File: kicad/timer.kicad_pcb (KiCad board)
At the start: 2 copper layers, 35.1 x 40 mm, 27 parts, among them IC1 STM8S003F3P, J1 PISK, J2 USB_OTG, J3 CONN_01X02, P1 kn1, P2 bat, P3 kn1, Q4 Q_NMOS_GSD, U1 TP4056

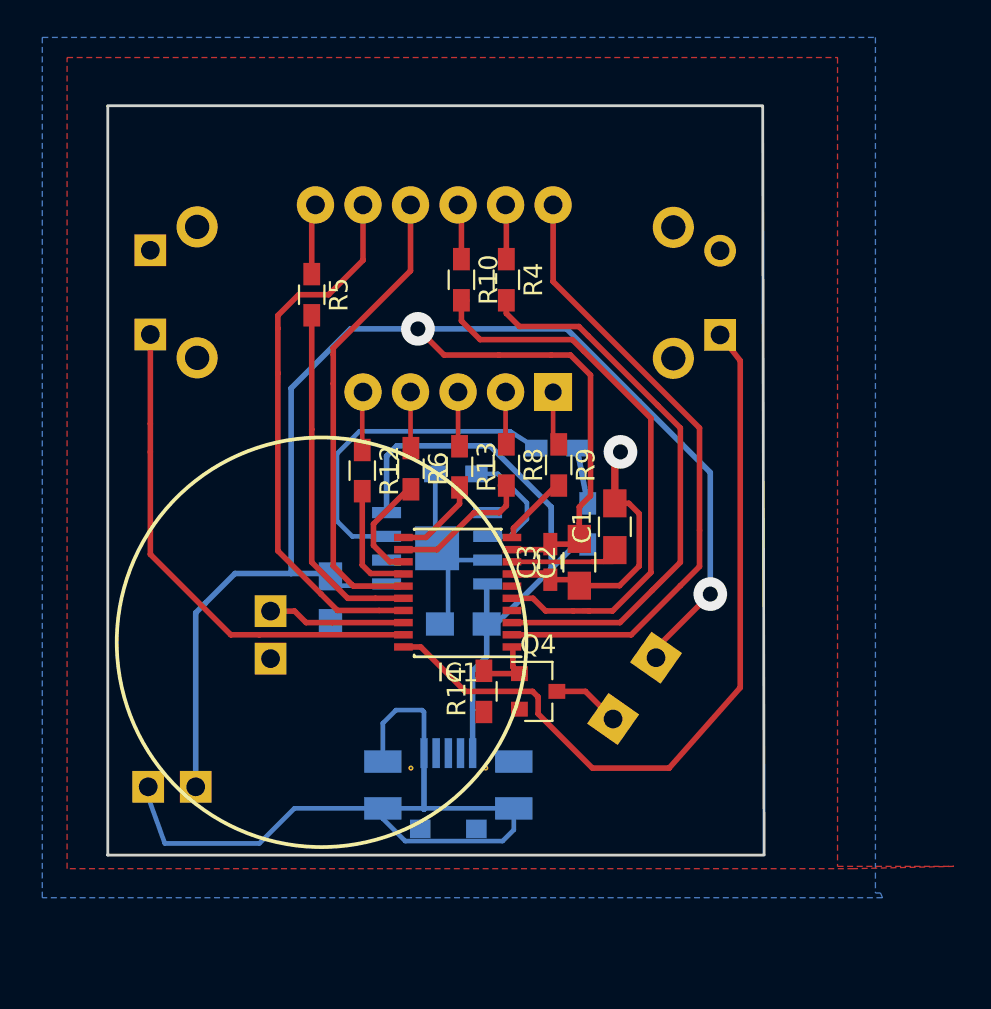
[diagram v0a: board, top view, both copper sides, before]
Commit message: start
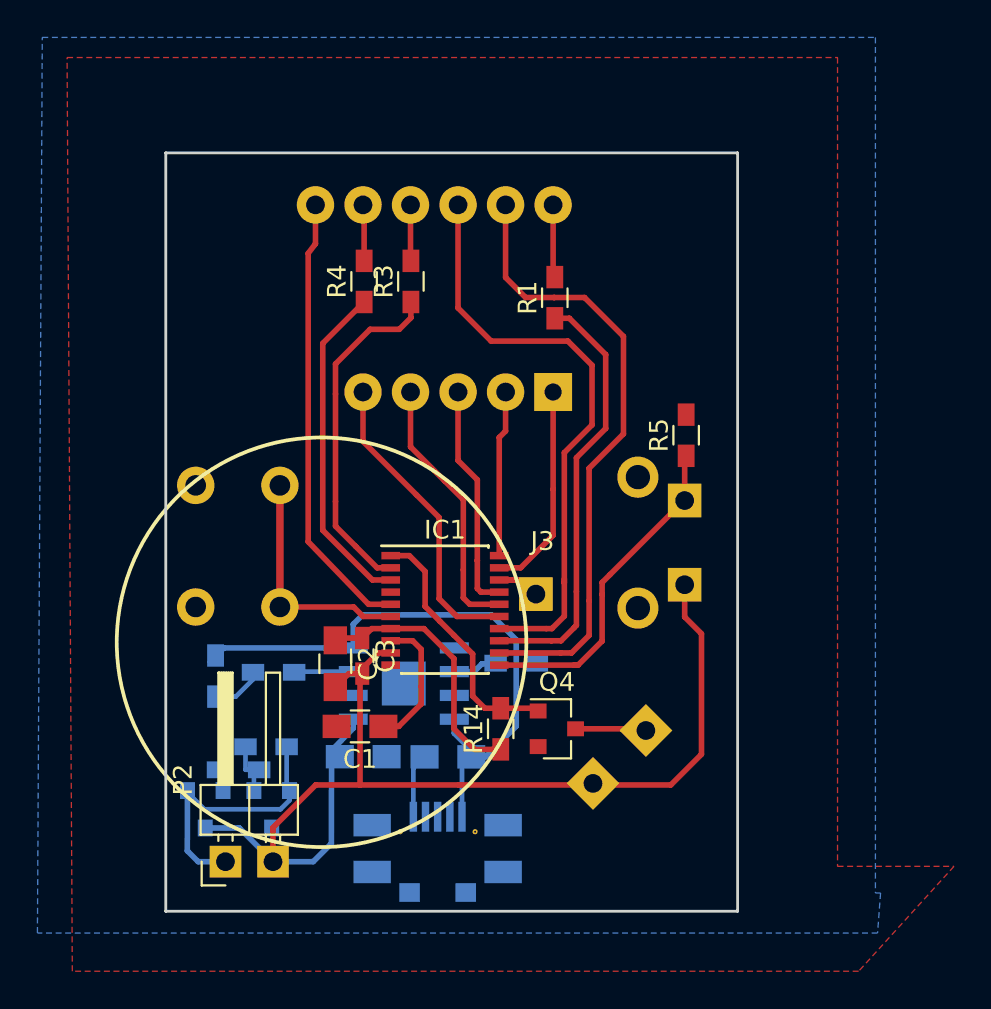
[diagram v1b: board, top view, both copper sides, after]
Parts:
- removed R10, R12, R13, R8, R9: 1k, Resistors_SMD:R_0603_HandSoldering
- added J4: max809, TO_SOT_Packages_SMD:SOT-23, B.Cu at (107.2, 82.3)
- added Q1: IRLML6244TRPBF, TO_SOT_Packages_SMD:SOT-23, B.Cu at (110.8, 82.3)
- added R1: 200, Resistors_SMD:R_0603_HandSoldering, F.Cu at (125.9, 55.0)
- added R3: 200, Resistors_SMD:R_0603_HandSoldering, F.Cu at (118.2, 54.1)
- added R7: 100k, Resistors_SMD:R_0603_HandSoldering, B.Cu at (110.5, 79.0)
- AFF1: footprint mylibpcb:indicator_3cif -> myowndevice:indicator_3cif
- J1: footprint mylibpcb:hc0903a -> myowndevice:hc0903a
- J2: footprint mylibpcb:usb5s -> myowndevice:usb5s
- J3: value CONN_01X02 -> Conn_01x01; footprint Pin_Headers:Pin_Header_Angled_1x02_Pitch2.54mm -> myowndevice:1pin_sq; moved to F.Cu
- P2: moved to F.Cu
- P3: footprint Buttons_Switches_THT:SW_Tactile_SKHH_Angled -> Buttons_Switches_ThroughHole:SW_PUSH_6mm_h8mm
- R2: value 10k -> 30k (40ma)
- R4: value 1k -> 200
- R5: value 1k -> 10k
- R6: moved to B.Cu
- moved D1 21.5 mm to (107.8, 75.2), turned to 90 degrees
- moved R5 21.4 mm to (132.9, 62.3), turned to 90 degrees
- moved R11 19.3 mm to (110.9, 75.0), turned to 0 degrees
- moved R6 18.5 mm to (109.0, 80.2), turned to 180 degrees
- moved C1 17.3 mm to (115.5, 77.9), turned to 180 degrees
- moved J3 14.6 mm to (124.9, 70.8)
- moved C2 14.1 mm to (114.2, 74.5), turned to 270 degrees
- moved P1 13.5 mm to (132.8, 70.3)
- moved P3 12.8 mm to (106.7, 65.0)
- moved C3 11.2 mm to (115.6, 74.1), turned to 270 degrees
- moved R2 10.6 mm to (123.8, 74.5), turned to 0 degrees
- moved C5 8.57 mm to (115.7, 79.5), turned to 0 degrees
- moved R4 7.60 mm to (115.7, 54.1), turned to 90 degrees
- moved U1 7.45 mm to (117.8, 75.6)
- moved C4 7.15 mm to (120.2, 79.5)
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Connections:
- AFF1 pad 1: Net-(AFF1-Pad1) -> /e
- AFF1 pad 10: Net-(AFF1-Pad10) -> /f
- AFF1 pad 11: Net-(AFF1-Pad11) -> /a
- AFF1 pad 12: /c1 -> Net-(AFF1-Pad12)
- AFF1 pad 2: Net-(AFF1-Pad2) -> /d
- AFF1 pad 3: Net-(AFF1-Pad3) -> /dp
- AFF1 pad 4: Net-(AFF1-Pad4) -> /c
- AFF1 pad 5: Net-(AFF1-Pad5) -> /g
- AFF1 pad 7: Net-(AFF1-Pad7) -> /b
- AFF1 pad 8: /c3 -> Net-(AFF1-Pad8)
- AFF1 pad 9: /c2 -> Net-(AFF1-Pad9)
- IC1 pad 10: /e -> (no net)
- IC1 pad 11: /dp -> /kn2
- IC1 pad 12: /d -> /a
- IC1 pad 13: /c -> /c1
- IC1 pad 14: /g -> /f
- IC1 pad 15: /c2 -> /g
- IC1 pad 16: /b -> /c
- IC1 pad 17: /c3 -> /dp
- IC1 pad 19: /kn -> /e
- IC1 pad 2: /c1 -> /c2
- IC1 pad 20: /kn2 -> /d
- IC1 pad 3: /a -> /c3
- IC1 pad 4: Net-(IC1-Pad4) -> (no net)
- IC1 pad 5: /f -> /b
- IC1 pad 6: Net-(IC1-Pad6) -> /kn
- J1 pad 1: VDD -> Net-(J1-Pad1)
- J1 pad 2: Net-(J1-Pad2) -> VDD
- J2 pad 2: Net-(J2-Pad2) -> (no net)
- J2 pad 3: Net-(J2-Pad3) -> (no net)
- J2 pad 4: Net-(J2-Pad4) -> (no net)
- J3 pad 1: GND -> /prg
- P1 pad 1: /kn2 -> VDD
- P1 pad 2: GND -> /kn2
- P2 pad 1: VDD -> Net-(J4-Pad1)
- P2 pad 2: GND -> VDD
- Q4 pad 3: Net-(J1-Pad2) -> Net-(J1-Pad1)
- R4 pad 1: Net-(AFF1-Pad11) -> /c3
- R4 pad 2: /a -> Net-(AFF1-Pad8)
- R5 pad 1: Net-(AFF1-Pad7) -> /kn2
- R5 pad 2: /b -> GND
- R6 pad 1: Net-(AFF1-Pad4) -> Net-(Q1-Pad1)
- R6 pad 2: /c -> Net-(J4-Pad2)
- U1 pad 1: Net-(U1-Pad1) -> GND
- U1 pad 6: Net-(U1-Pad6) -> (no net)
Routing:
- net GND: track 66.3 -> 17.9 mm, vias 1 -> 0
- net VDD: track 91.7 -> 61.2 mm, vias 2 -> 0
- net /kn2: track 42.6 -> 17.8 mm
- net Net-(R11-Pad2): track 18.0 -> 3.17 mm
- net Net-(J4-Pad1): track 0.00 -> 14.8 mm
- net /kn: track 27.1 -> 12.6 mm
- net /c1: track 35.5 -> 23.5 mm
- net /c3: track 29.8 -> 17.8 mm
- net /pisk: track 3.53 -> 13.7 mm
- net /g: track 6.40 -> 16.3 mm
- net /c: track 6.27 -> 14.2 mm
- net /e: track 3.87 -> 11.3 mm
- net /dp: track 5.02 -> 12.2 mm
- net /c2: track 25.8 -> 18.8 mm
- net /b: track 18.8 -> 24.0 mm
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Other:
- board size 35.1 x 40 mm -> 30.6 x 40.5 mm
